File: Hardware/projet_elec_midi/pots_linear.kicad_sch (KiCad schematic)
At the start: 18 parts, among them U7 74HC4051

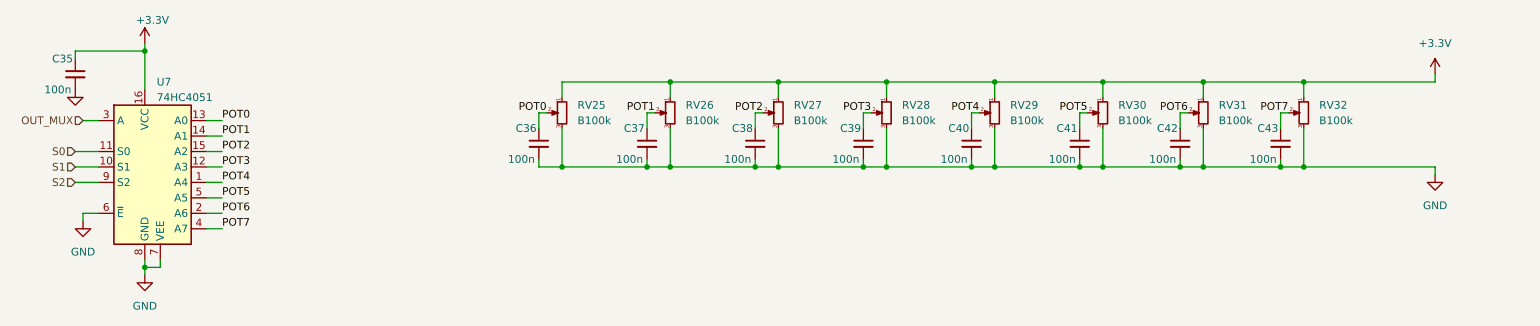
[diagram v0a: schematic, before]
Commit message: Kicad schematic terminée
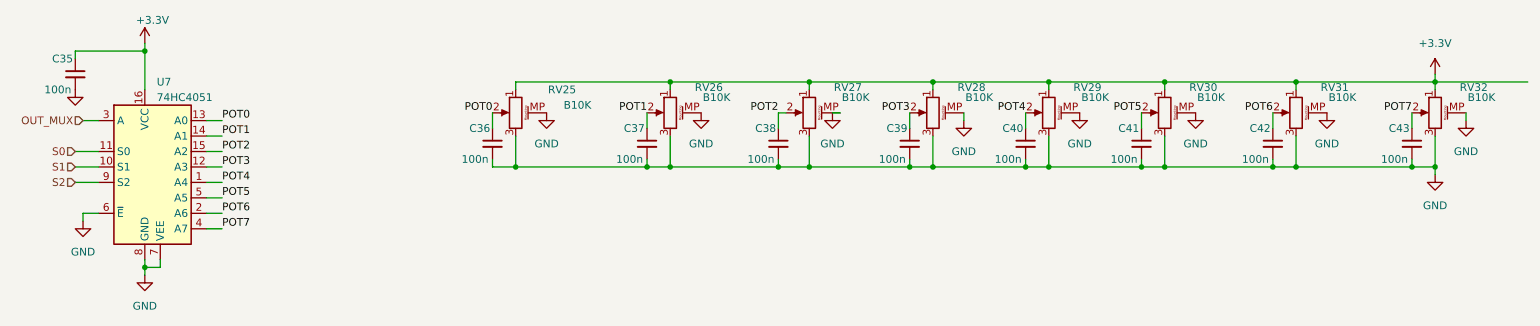
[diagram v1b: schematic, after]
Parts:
- removed RV25, RV26, RV27, RV28, RV29, RV30, RV31, RV32: B100k, Potentiometer_THT:Potentiometer_Bourns_PTA3043_Single_Slide, symbol Device:R_Potentiometer_Small
- added RV25, RV26, RV27, RV28, RV29, RV30, RV31, RV32: B10K, Potentiometer_THT:Potentiometer_Bourns_PTA3043_Single_Slide, symbol Device:R_Potentiometer_MountingPin
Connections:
- net +3.3V: now also RV25.1, RV26.1, RV27.1, RV28.1, RV29.1, RV30.1, RV31.1, RV32.1
- net GND: now also RV25.3, RV25.MP (MountPin), RV26.3, RV26.MP (MountPin), RV27.3, RV27.MP (MountPin), RV28.3, RV28.MP (MountPin), RV29.3, RV29.MP (MountPin), RV30.3, RV30.MP (MountPin), RV31.3, RV31.MP (MountPin), RV32.3, RV32.MP (MountPin)
- net POT0: now also RV25.2
- net POT1: now also RV26.2
- net POT2: now also RV27.2
- net POT3: now also RV28.2
- net POT4: now also RV29.2
- net POT5: now also RV30.2
- net POT6: now also RV31.2
- net POT7: now also RV32.2
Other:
- moved on the sheet: C36, C38, C39, C40, C41, C42, C43
